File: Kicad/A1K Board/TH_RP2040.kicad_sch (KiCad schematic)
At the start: 13 parts, among them U1 RP2040, U3 W25Q16JVSS, Y1 12MHz

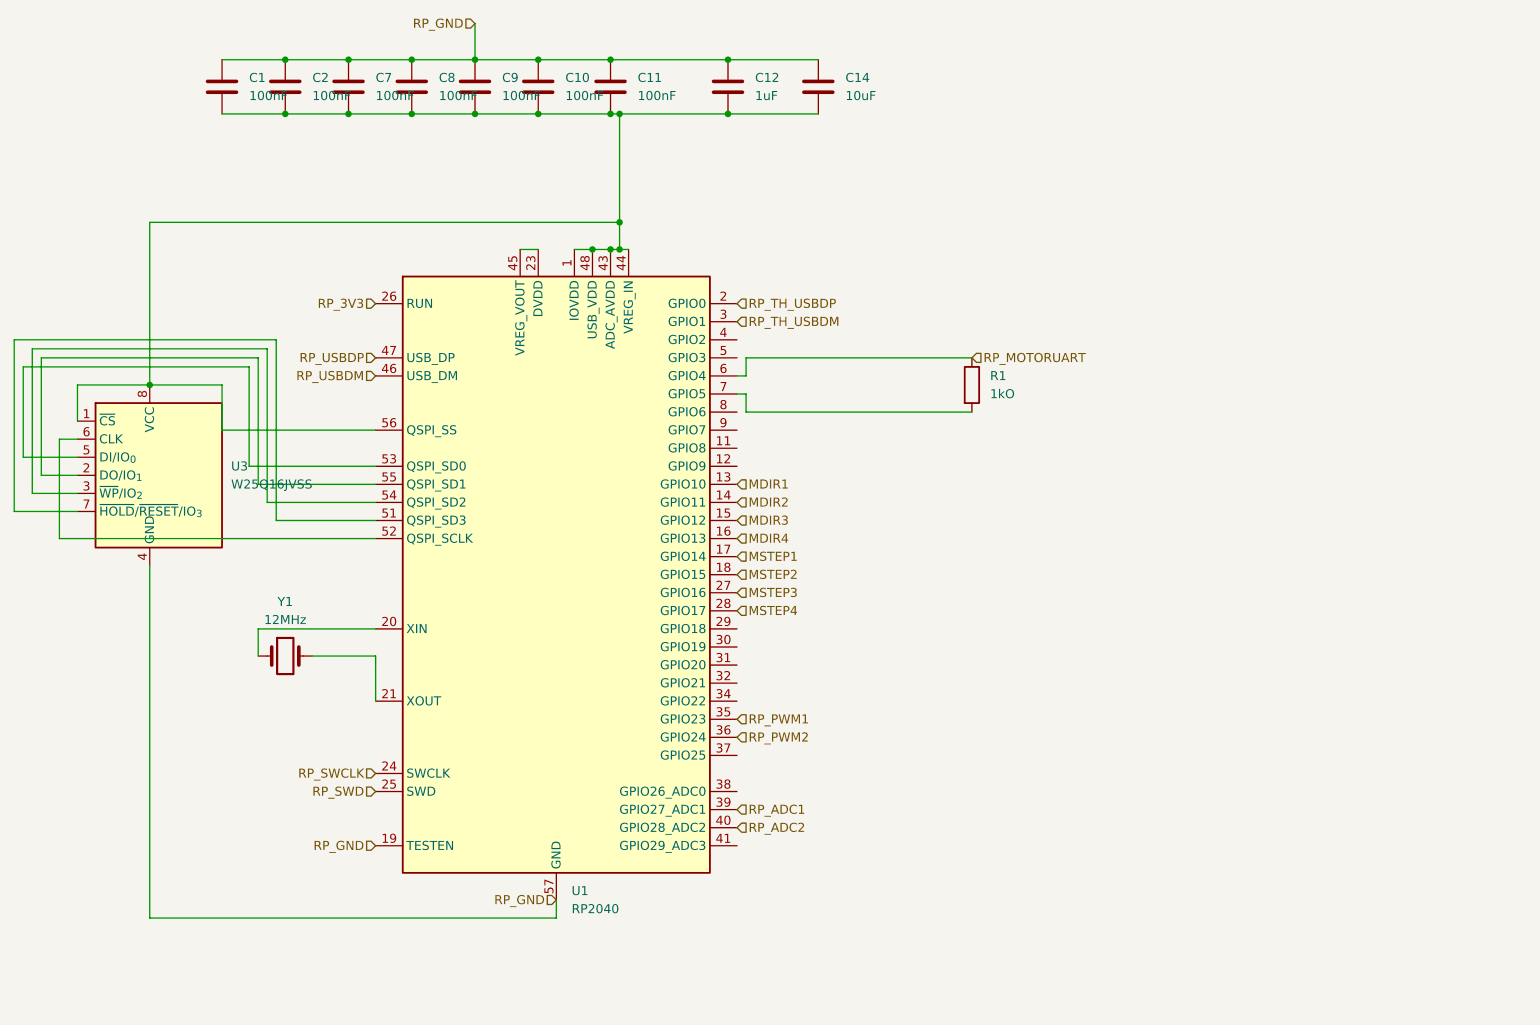
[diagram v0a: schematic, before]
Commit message: e
e
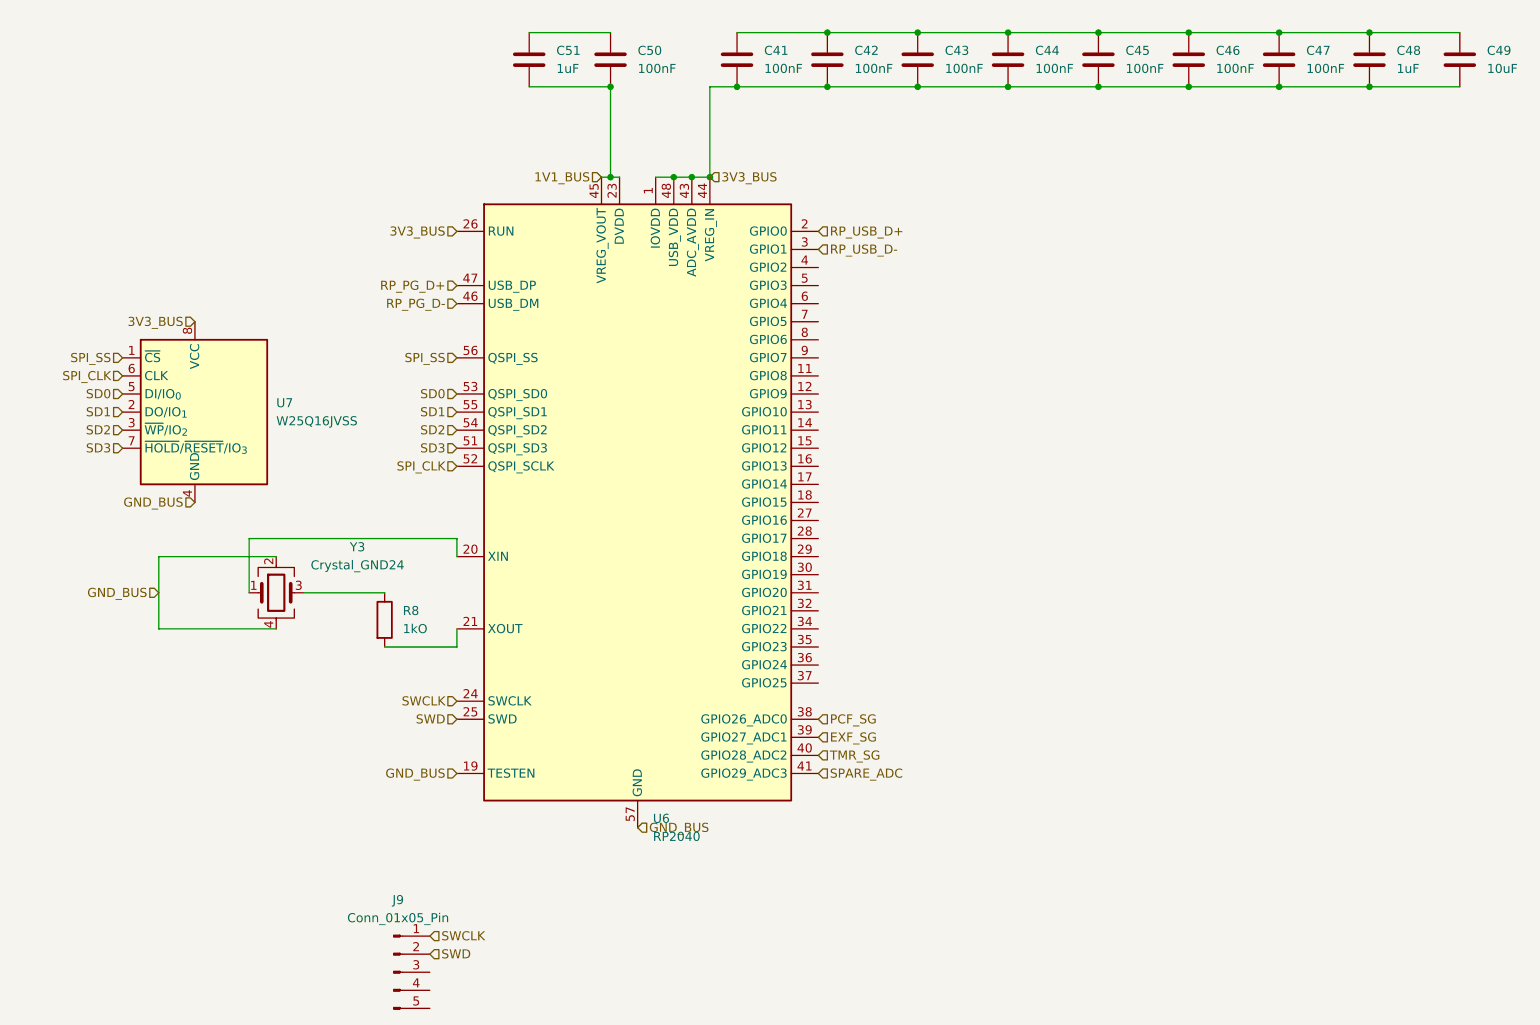
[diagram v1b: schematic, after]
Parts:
- removed C1, C10, C11, C2, C7, C8, C9: 100nF, symbol Device:C
- removed C12: 1uF, symbol Device:C
- removed C14: 10uF, symbol Device:C
- removed R1: 1kO, symbol Device:R
- removed U1: RP2040, Package_DFN_QFN:QFN-56-1EP_7x7mm_P0.4mm_EP3.2x3.2mm, symbol MCU_RaspberryPi:RP2040
- removed U3: W25Q16JVSS, Package_SO:SOIC-8_5.3x5.3mm_P1.27mm, symbol Memory_Flash:W25Q16JVSS
- removed Y1: 12MHz, symbol Device:Crystal
- added C41, C42, C43, C44, C45, C46, C47, C50: 100nF, Capacitor_SMD:C_0402_1005Metric, symbol Device:C
- added C48, C51: 1uF, Capacitor_SMD:C_0603_1608Metric, symbol Device:C
- added C49: 10uF, Capacitor_SMD:C_0603_1608Metric, symbol Device:C
- added J9: Conn_01x05_Pin, Connector_PinHeader_2.54mm:PinHeader_1x05_P2.54mm_Vertical, symbol Connector:Conn_01x05_Pin
- added R8: 1kO, Resistor_SMD:R_1206_3216Metric, symbol Device:R
- added U6: RP2040, Package_DFN_QFN:QFN-56-1EP_7x7mm_P0.4mm_EP3.2x3.2mm, symbol MCU_RaspberryPi:RP2040
- added U7: W25Q16JVSS, Package_SO:SOIC-8_5.3x5.3mm_P1.27mm, symbol Memory_Flash:W25Q16JVSS
- added Y3: Crystal_GND24, Crystal:Crystal_SMD_3225-4Pin_3.2x2.5mm, symbol Device:Crystal_GND24
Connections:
- new net: C41.1, C42.1, C43.1, C44.1, C45.1, C46.1, C47.1, C48.1, C49.1
- new net: U6.20 (XIN), Y3.1
- new net: R8.1, Y3.3
- new net: C50.1, C51.1
- new net: R8.2, U6.21 (XOUT)
- new net 1V1_BUS: C50.2, C51.2, U6.23 (DVDD), U6.45 (VREG_VOUT), U6.50 (DVDD)
- new net 3V3_BUS: C41.2, C42.2, C43.2, C44.2, C45.2, C46.2, C47.2, C48.2, C49.2, U6.1 (IOVDD), U6.10 (IOVDD), U6.22 (IOVDD), U6.26 (RUN), U6.33 (IOVDD), U6.42 (IOVDD), U6.43 (ADC_AVDD), U6.44 (VREG_IN), U6.48 (USB_VDD), U6.49 (IOVDD), U7.8 (VCC)
- new net EXF_SG: U6.39 (GPIO27_ADC1)
- new net GND_BUS: U6.19 (TESTEN), U6.57 (GND), U7.4 (GND), Y3.2, Y3.4
- new net PCF_SG: U6.38 (GPIO26_ADC0)
- new net RP_PG_D+: U6.47 (USB_DP)
- new net RP_PG_D-: U6.46 (USB_DM)
- new net RP_USB_D+: U6.2 (GPIO0)
- new net RP_USB_D-: U6.3 (GPIO1)
- new net SD0: U6.53 (QSPI_SD0), U7.5 (DI/IO_{0})
- new net SD1: U6.55 (QSPI_SD1), U7.2 (DO/IO_{1})
- new net SD2: U6.54 (QSPI_SD2), U7.3 (~{WP}/IO_{2})
- new net SD3: U6.51 (QSPI_SD3), U7.7 (~{HOLD}/~{RESET}/IO_{3})
- new net SPARE_ADC: U6.41 (GPIO29_ADC3)
- new net SPI_CLK: U6.52 (QSPI_SCLK), U7.6 (CLK)
- new net SPI_SS: U6.56 (QSPI_SS), U7.1 (~{CS})
- new net SWCLK: J9.1 (Pin_1), U6.24 (SWCLK)
- new net SWD: J9.2 (Pin_2), U6.25 (SWD)
- new net TMR_SG: U6.40 (GPIO28_ADC2)
